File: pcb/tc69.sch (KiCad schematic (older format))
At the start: 95 parts, among them SW1 ESC, SW10 LWIN, SW11 2, SW12 W, SW13 A, SW14 Z, SW16 3, SW17 E, SW18 S, SW19 X, SW2 TAB, SW20 LALT, SW21 4, SW22 R, SW23 D, SW24 C, SW26 5, SW27 T, SW28 F, SW29 V, SW3 CAPS, SW30 LSPC, SW31 6, SW32 Y, SW33 G, SW34 B, SW36 7, SW37 U, SW38 H, SW39 N, SW41 8, SW42 I, SW43 J, SW44 M, SW45 RSPC, SW46 9, SW47 O, SW48 K, SW49 COMMA, SW5 LCTRL, SW51 0, SW52 P, SW53 L, SW54 DOT, SW55 RALT, SW56 MINUS, SW57 LBRC, SW58 SCLN, SW59 SLSH, SW6 1, SW60 RWIN, SW61 EQUAL, SW62 RBRC, SW63 QUOTE, SW65 APP, SW66 BS, SW68 ENTER, SW69 RSHFT, SW7 Q, SW70 LEFT, SW72 BSLSH, SW74 UP, SW75 DOWN, SW76 HOME, SW77 PGUP, SW78 PGDN, SW79 END, SW80 RIGHT, SW9 LSHFT, U1 SeeeduinoXIAO, U2 CD74HC4067SM, U3 TLV9051

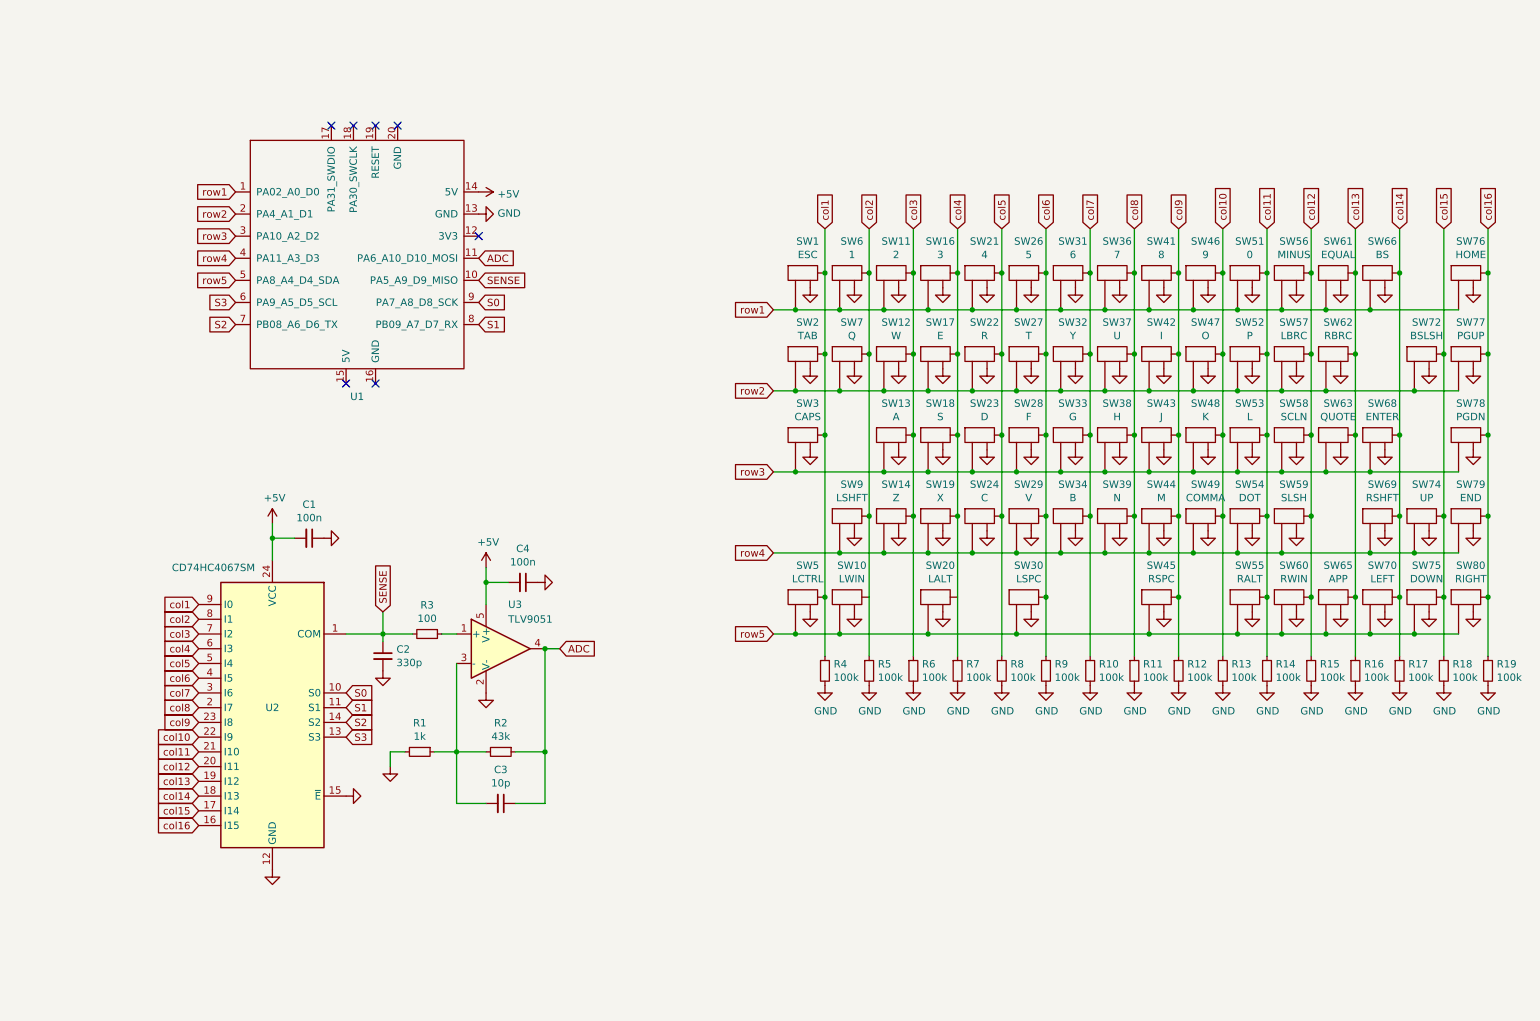
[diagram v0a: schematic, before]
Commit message: wire a bit
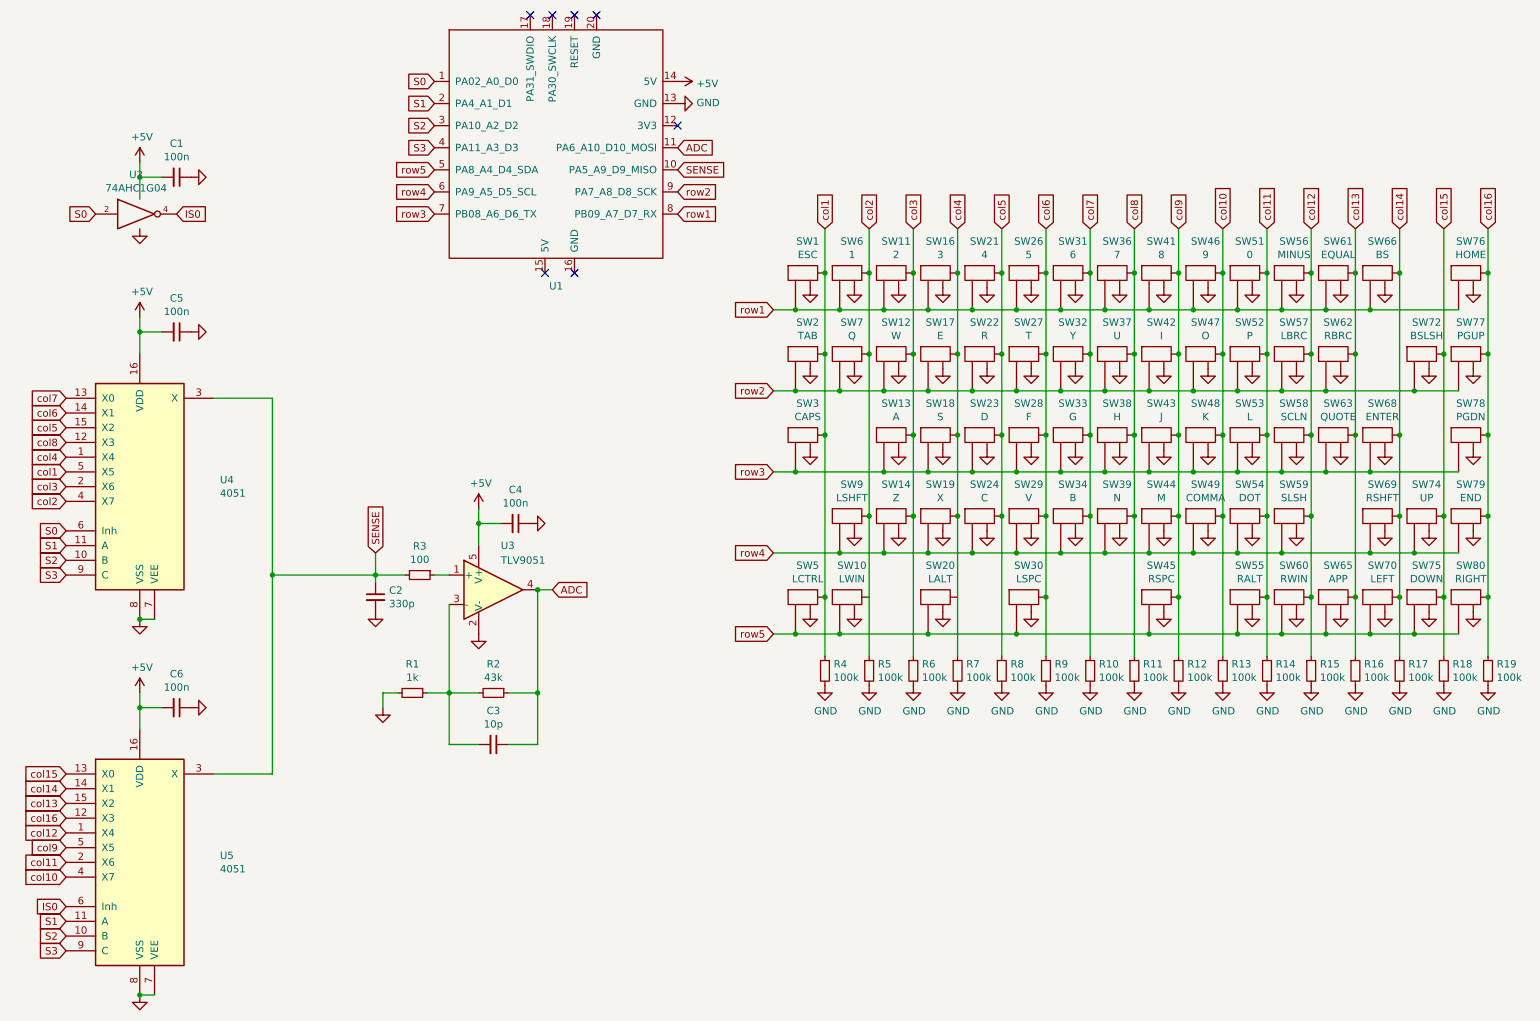
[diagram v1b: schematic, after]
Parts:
- removed U2: CD74HC4067SM, Package_SO:SSOP-24_5.3x8.2mm_P0.65mm, symbol 74xx:CD74HC4067SM
- added C5, C6: 100n, Capacitor_SMD:C_0402_1005Metric, symbol Device:C_Small
- added U2: 74AHC1G04, Package_TO_SOT_SMD:SOT-23-5, symbol 74xGxx:74AHC1G04
- added U4, U5: 4051, Package_SO:SOIC-16_3.9x9.9mm_P1.27mm, symbol 4xxx:4051
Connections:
- net +5V: now also C5.2, C6.2, U2.5 (VCC), U4.16 (VDD), U5.16 (VDD)
- net GND: now also C5.1, C6.1, U2.3 (GND), U4.7 (VEE), U4.8 (VSS), U5.7 (VEE), U5.8 (VSS)
- net S0: now also U1.1 (PA02_A0_D0), U2.2, U4.6 (Inh); no longer U1.9 (PA7_A8_D8_SCK)
- net S1: now also U1.2 (PA4_A1_D1), U4.11 (A), U5.11 (A); no longer U1.8 (PB09_A7_D7_RX)
- net S2: now also U1.3 (PA10_A2_D2), U4.10 (B), U5.10 (B); no longer U1.7 (PB08_A6_D6_TX)
- net S3: now also U1.4 (PA11_A3_D3), U4.9 (C), U5.9 (C); no longer U1.6 (PA9_A5_D5_SCL)
- net SENSE: now also U4.3 (X), U5.3 (X)
- net col1: now also U4.5 (X5)
- net col10: now also U5.4 (X7)
- net col11: now also U5.2 (X6)
- net col12: now also U5.1 (X4)
- net col13: now also U5.15 (X2)
- net col14: now also U5.14 (X1)
- net col15: now also U5.13 (X0)
- net col16: now also U5.12 (X3)
- net col2: now also U4.4 (X7)
- net col3: now also U4.2 (X6)
- net col4: now also U4.1 (X4)
- net col5: now also U4.15 (X2)
- net col6: now also U4.14 (X1)
- net col7: now also U4.13 (X0)
- net col8: now also U4.12 (X3)
- net col9: now also U5.5 (X5)
- net row1: now also U1.8 (PB09_A7_D7_RX); no longer U1.1 (PA02_A0_D0)
- net row2: now also U1.9 (PA7_A8_D8_SCK); no longer U1.2 (PA4_A1_D1)
- net row3: now also U1.7 (PB08_A6_D6_TX); no longer U1.3 (PA10_A2_D2)
- net row4: now also U1.6 (PA9_A5_D5_SCL); no longer U1.4 (PA11_A3_D3)
- new net IS0: U2.4, U5.6 (Inh)
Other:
- moved on the sheet: C1, C2, C3, C4, R1, R2, R3, U1, U3
